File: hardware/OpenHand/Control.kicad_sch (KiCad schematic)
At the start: 3 parts, among them U3 DRV8833PWP, U4 DRV8833PWP, U5 DRV8833PWP

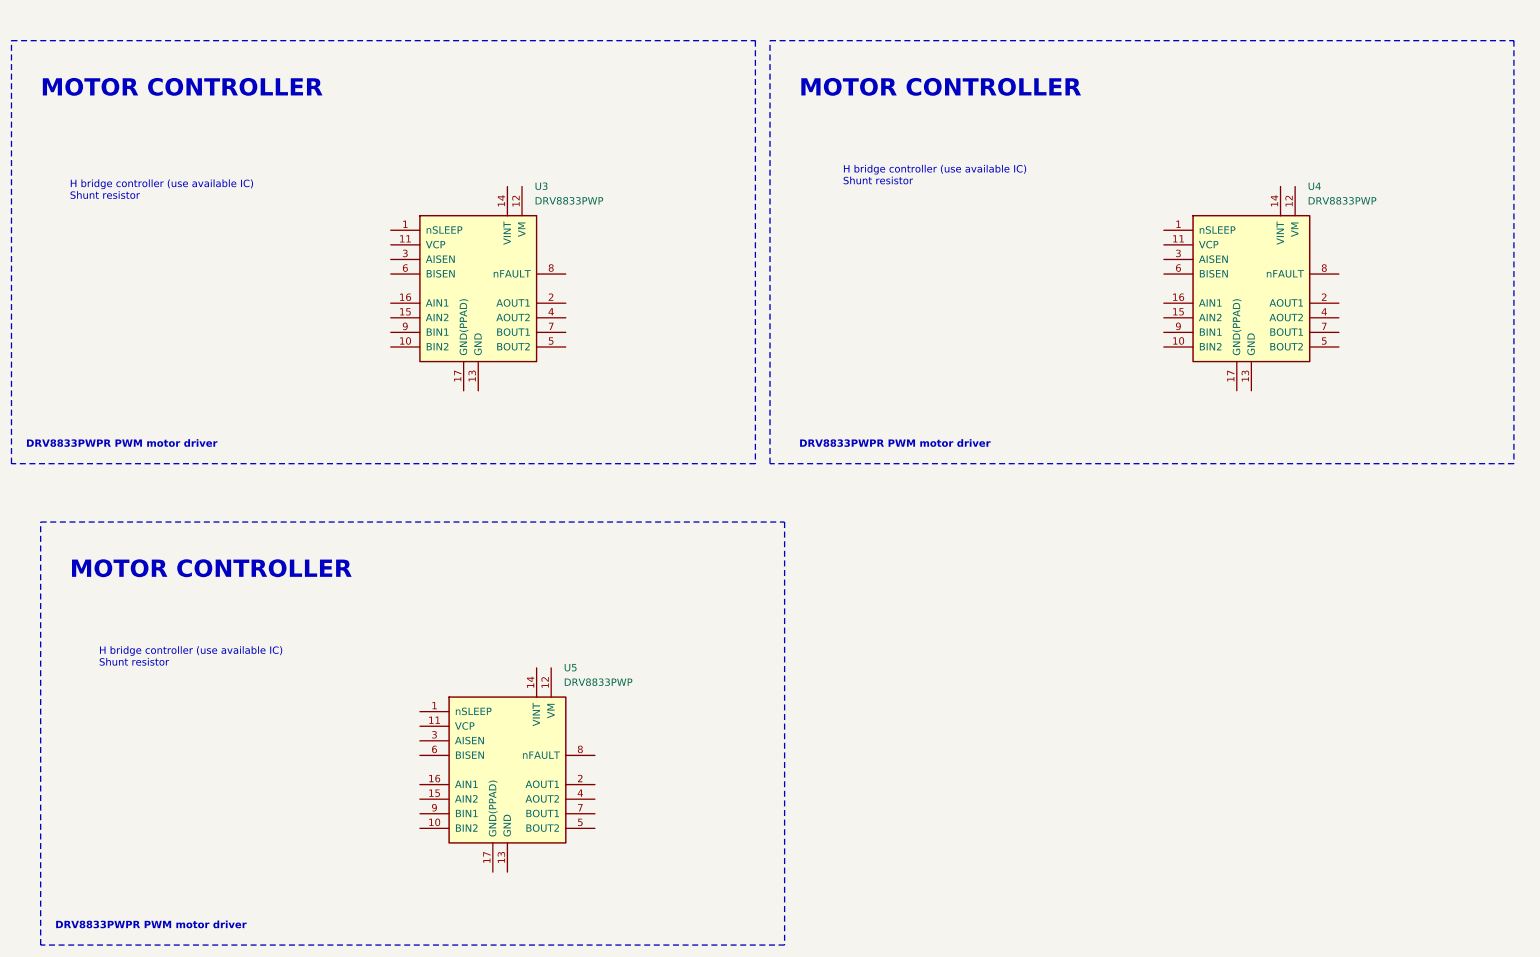
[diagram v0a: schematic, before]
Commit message: Update schematic
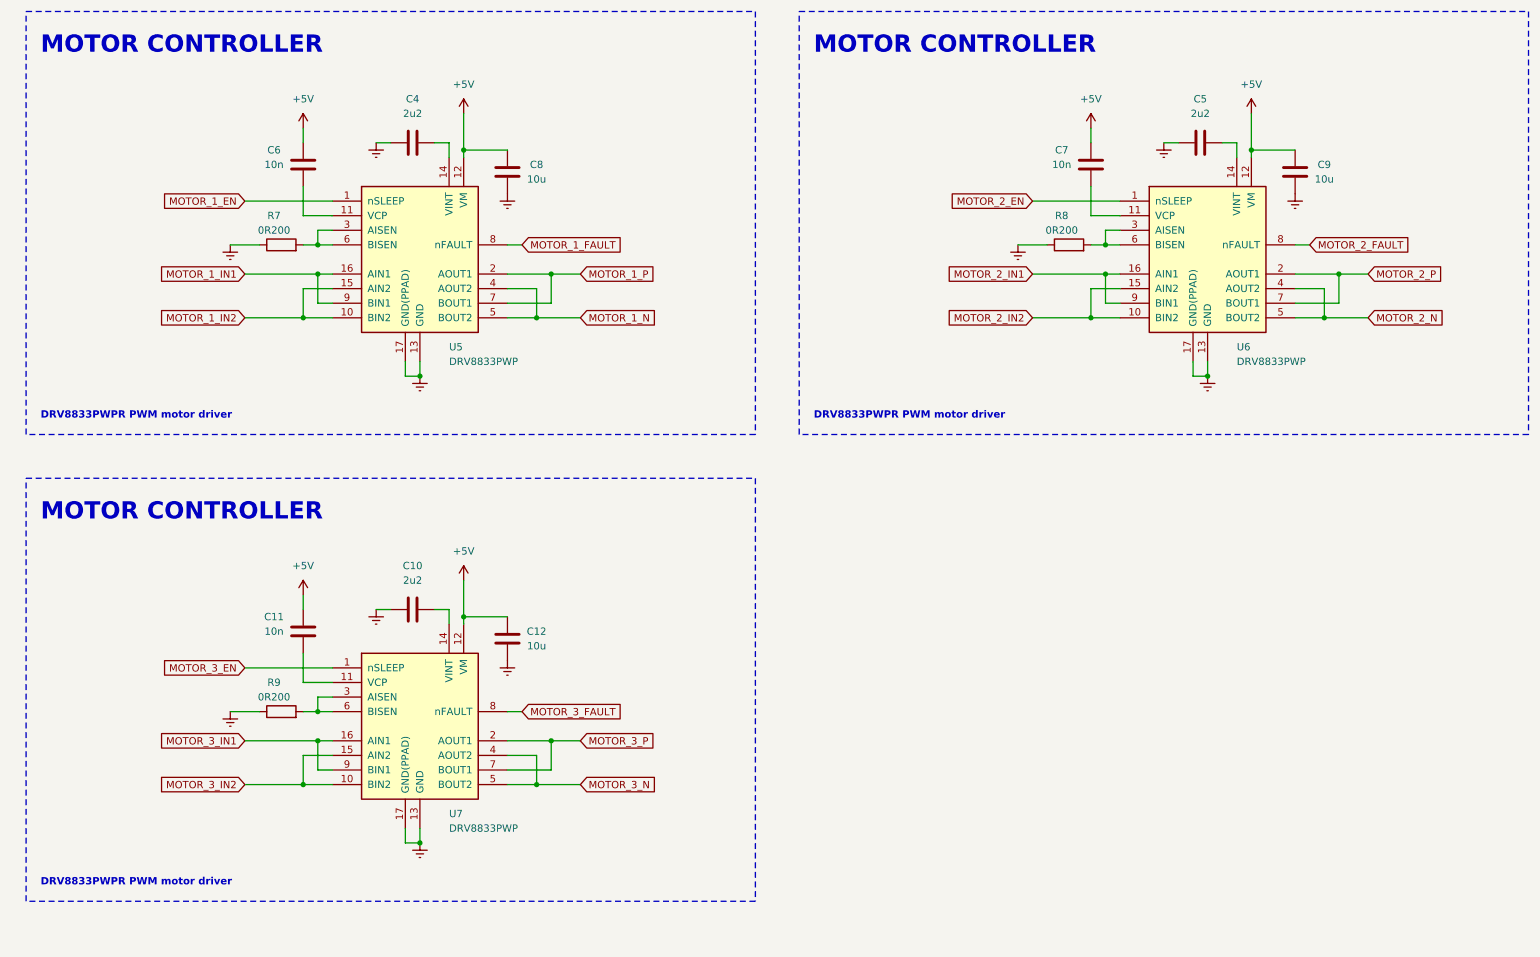
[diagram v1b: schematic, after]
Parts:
- removed U3, U4: DRV8833PWP, Package_SO:HTSSOP-16-1EP_4.4x5mm_P0.65mm_EP3.4x5mm_Mask2.46x2.31mm_ThermalVias, symbol Driver_Motor:DRV8833PWP
- added C10, C4, C5: 2u2, symbol Device:C
- added C11, C6, C7: 10n, symbol Device:C
- added C12, C8, C9: 10u, symbol Device:C
- added R7, R8, R9: 0R200, symbol Device:R
- added U5, U6: DRV8833PWP, Package_SO:HTSSOP-16-1EP_4.4x5mm_P0.65mm_EP3.4x5mm_Mask2.46x2.31mm_ThermalVias, symbol Driver_Motor:DRV8833PWP
- renumbered U5 to U7
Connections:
- net MOTOR_3_EN: now reaches U7.1 (nSLEEP)
- net MOTOR_3_IN2: now reaches U7.10 (BIN2)
- net MOTOR_3_IN2: now also U7.15 (AIN2)
- net at U7.11 (VCP): now also C11.2
- net +5V: now reaches U7.12 (VM)
- net +5V: now also C11.1, C12.1, C6.1, C7.1, C8.1, C9.1, U5.12 (VM), U6.12 (VM)
- net Earth: now reaches U7.13 (GND)
- net Earth: now also U7.17 (GND(PPAD)), C10.1, C12.2, C4.1, C5.1, C8.2, C9.2, R7.1, R8.1, R9.1, U5.13 (GND), U5.17 (GND(PPAD)), U6.13 (GND), U6.17 (GND(PPAD))
- net at U7.14 (VINT): now also C10.2
- net MOTOR_3_IN1: now reaches U7.16 (AIN1)
- net MOTOR_3_IN1: now also U7.9 (BIN1)
- net MOTOR_3_P: now reaches U7.2 (AOUT1)
- net MOTOR_3_P: now also U7.7 (BOUT1)
- net at U7.3 (AISEN): now also U7.6 (BISEN), R9.2
- net MOTOR_3_N: now reaches U7.4 (AOUT2)
- net MOTOR_3_N: now also U7.5 (BOUT2)
- net MOTOR_3_FAULT: now reaches U7.8 (nFAULT)
- new net: C7.2, U6.11 (VCP)
- new net: C5.2, U6.14 (VINT)
- new net: R8.2, U6.3 (AISEN), U6.6 (BISEN)
- new net: C6.2, U5.11 (VCP)
- new net: C4.2, U5.14 (VINT)
- new net: R7.2, U5.3 (AISEN), U5.6 (BISEN)
- new net MOTOR_1_EN: U5.1 (nSLEEP)
- new net MOTOR_1_FAULT: U5.8 (nFAULT)
- new net MOTOR_1_IN1: U5.16 (AIN1), U5.9 (BIN1)
- new net MOTOR_1_IN2: U5.10 (BIN2), U5.15 (AIN2)
- new net MOTOR_1_N: U5.4 (AOUT2), U5.5 (BOUT2)
- new net MOTOR_1_P: U5.2 (AOUT1), U5.7 (BOUT1)
- new net MOTOR_2_EN: U6.1 (nSLEEP)
- new net MOTOR_2_FAULT: U6.8 (nFAULT)
- new net MOTOR_2_IN1: U6.16 (AIN1), U6.9 (BIN1)
- new net MOTOR_2_IN2: U6.10 (BIN2), U6.15 (AIN2)
- new net MOTOR_2_N: U6.4 (AOUT2), U6.5 (BOUT2)
- new net MOTOR_2_P: U6.2 (AOUT1), U6.7 (BOUT1)
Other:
- note removed: "H bridge controller (use available IC) Shunt resistor"
- moved on the sheet: U7
